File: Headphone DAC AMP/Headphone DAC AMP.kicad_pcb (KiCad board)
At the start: 4 copper layers, 66.6 x 101.6 mm, 159 parts, among them J1 2137160001, J2 M50-3551042, J3 SJ-3502-SMT, J4 PINHD_1x2_Male, J5 PINHD_2x3_Male, U1 ES9039Q2M, U11 ADP5071AREZ-R7, U12 TPS74501PDRVR, U14 ADP7185ACPZN-R7, U2 XU316-1024-QF60B-C24, U3 TPA6120A2DWP, U4 OPA1612AxD, U5 OPA1612AxD, U6 MCP1727-1802xSN, U7 MCP1727-3302xSN, U8 W25Q16JVSNIQ, U9 TPS717XX, Y1 Crystal_GND24, Y2 LMK6CE049152CDLFR, Y3 ASDLJ-E-45.1584MHz

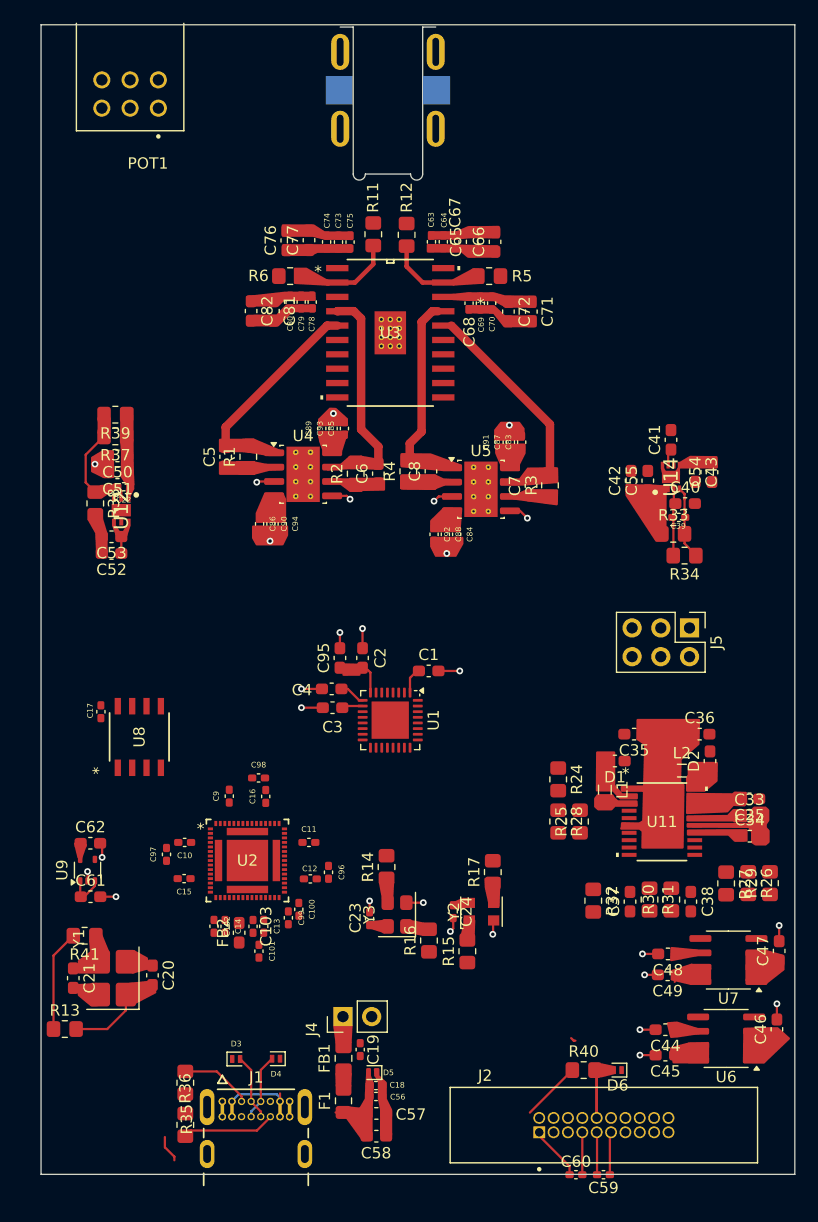
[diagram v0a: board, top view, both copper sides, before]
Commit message: Minor PCB Updates
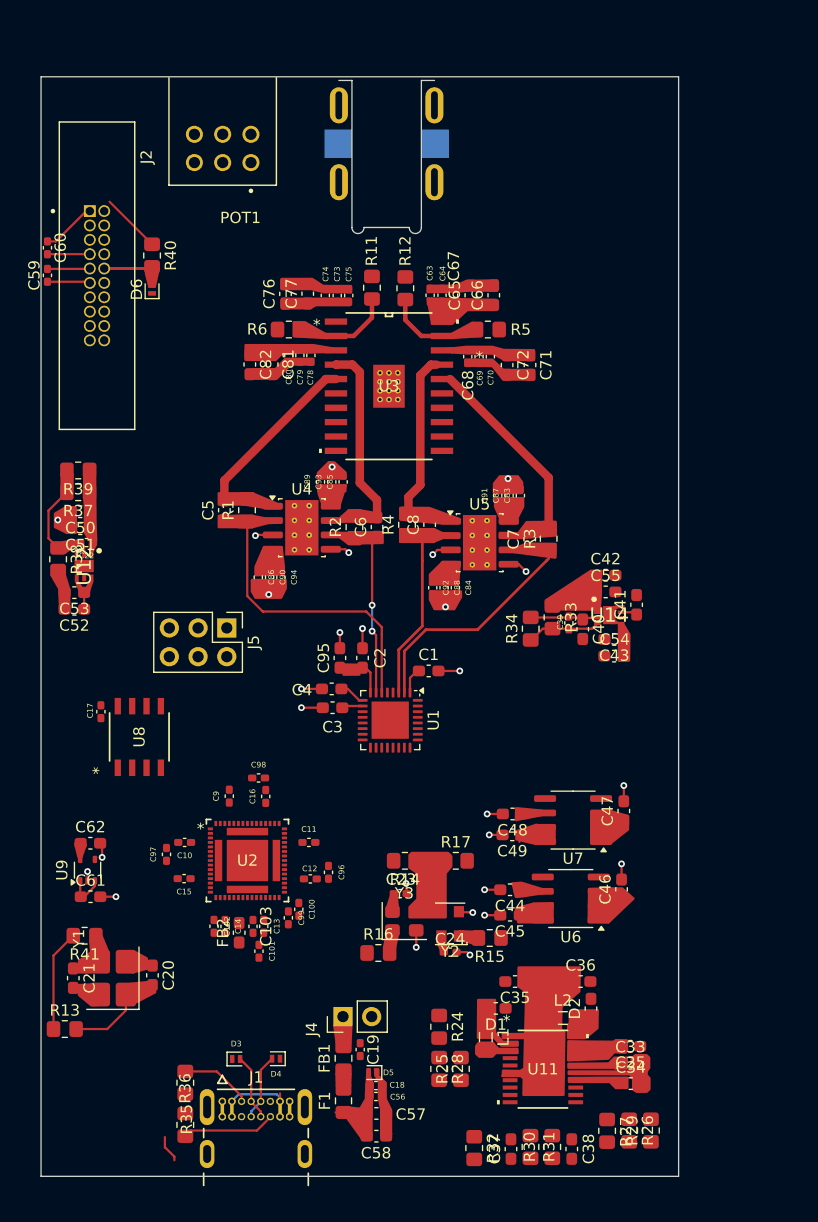
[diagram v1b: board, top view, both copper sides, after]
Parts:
- moved C60 94.3 mm to (79.4, 67.8), turned to -90 degrees
- moved C59 93.5 mm to (79.4, 70.2), turned to 90 degrees
- moved J2 87.5 mm to (83.8, 70.3), turned to -90 degrees
- moved R40 81.5 mm to (88.6, 68.5), turned to -90 degrees
- moved D6 80.4 mm to (88.6, 71.5), turned to 90 degrees
- moved J5 40.9 mm to (95.2, 101.4)
- moved C34 24.3 mm to (131.0, 141.7)
- moved C25 24.3 mm to (130.9, 138.4)
- moved C33 24.3 mm to (130.9, 139.9)
- moved C35 24.3 mm to (120.7, 132.7)
- moved L1 24.3 mm to (118.2, 137.6)
- moved L2 24.3 mm to (125.0, 135.9)
- moved R24 24.3 mm to (114.0, 136.7)
- moved R27 24.3 mm to (128.9, 145.9)
- moved R28 24.3 mm to (114.0, 140.4)
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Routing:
- net /DAC2-: track 0.00 -> 27.4 mm
- net /DAC1-: track 0.00 -> 20.6 mm
- net /DAC1+: track 0.00 -> 14.9 mm
- net /DAC2+: track 0.00 -> 14.1 mm, vias 0 -> 2
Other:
- board size 66.6 x 101.6 mm -> 56.4 x 97.2 mm
